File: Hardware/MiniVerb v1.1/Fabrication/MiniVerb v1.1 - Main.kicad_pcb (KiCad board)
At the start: 2 copper layers, 85 x 128.5 mm, 59 parts, among them J1 IDC_2x05, U1 TL074, U2 TL074

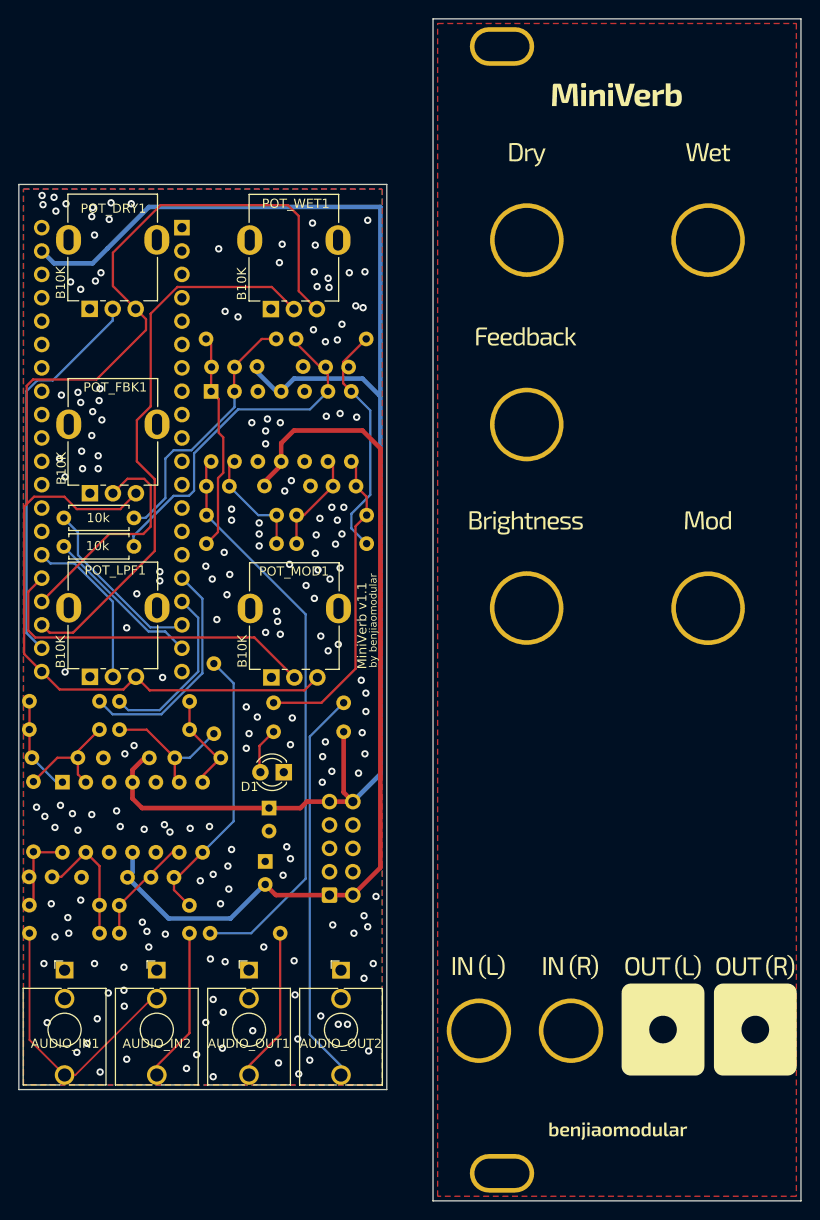
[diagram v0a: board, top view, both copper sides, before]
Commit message: Added BOM
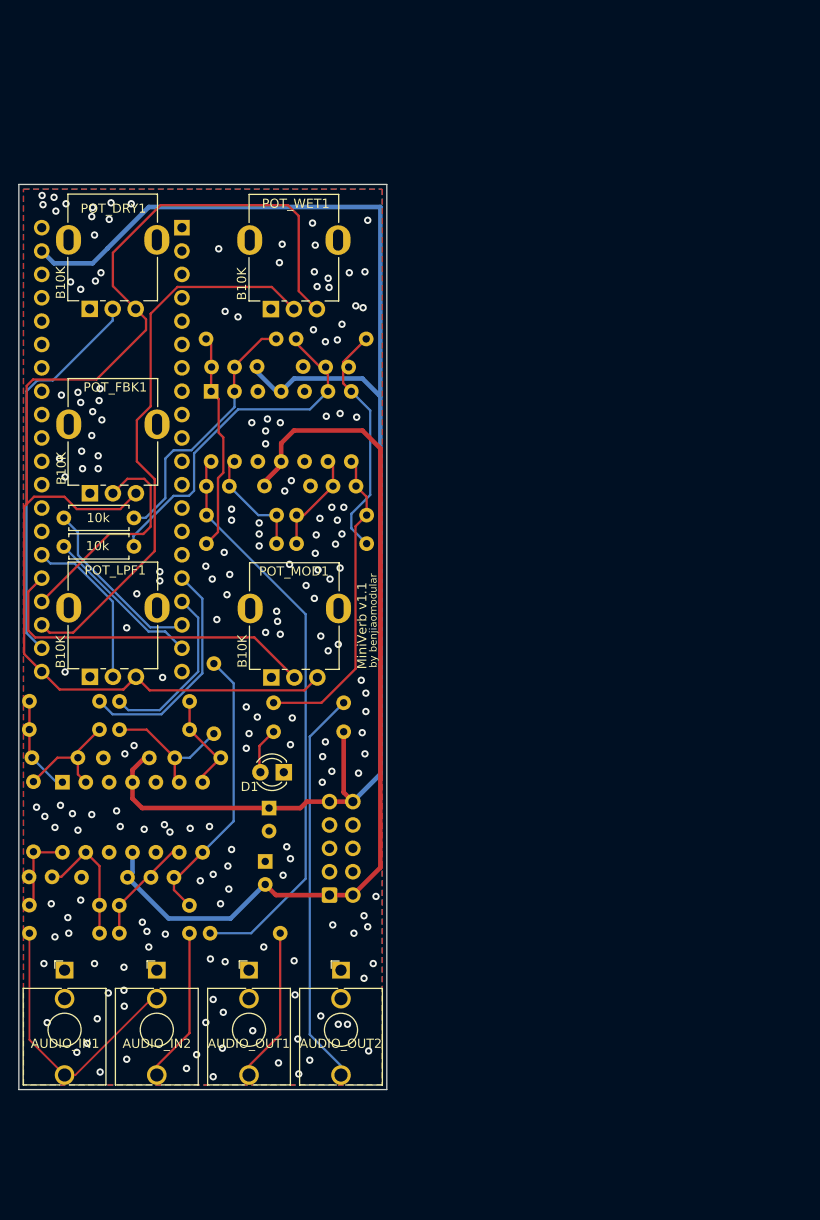
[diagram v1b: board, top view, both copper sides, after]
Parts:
- removed REF**: Panel_8HP, benjiaomodular:Panel_8HP
- removed REF** (x4): PanelHole_AudioJack_3.5mm, benjiaomodular:PanelHole_AudioJack_3.5mm
- removed REF** (x5): PanelHole_Potentiometer_RV09, benjiaomodular:PanelHole_Potentiometer_RV09
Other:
- board size 85 x 128.5 mm -> 40 x 98.4 mm
